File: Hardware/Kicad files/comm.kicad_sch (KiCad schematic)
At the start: 5 parts, among them J301 M80-5402642, J302 Conn_02x25_Top_Bottom, U301 MAX485_MODULE_5V_LOGIC_TLL_TO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

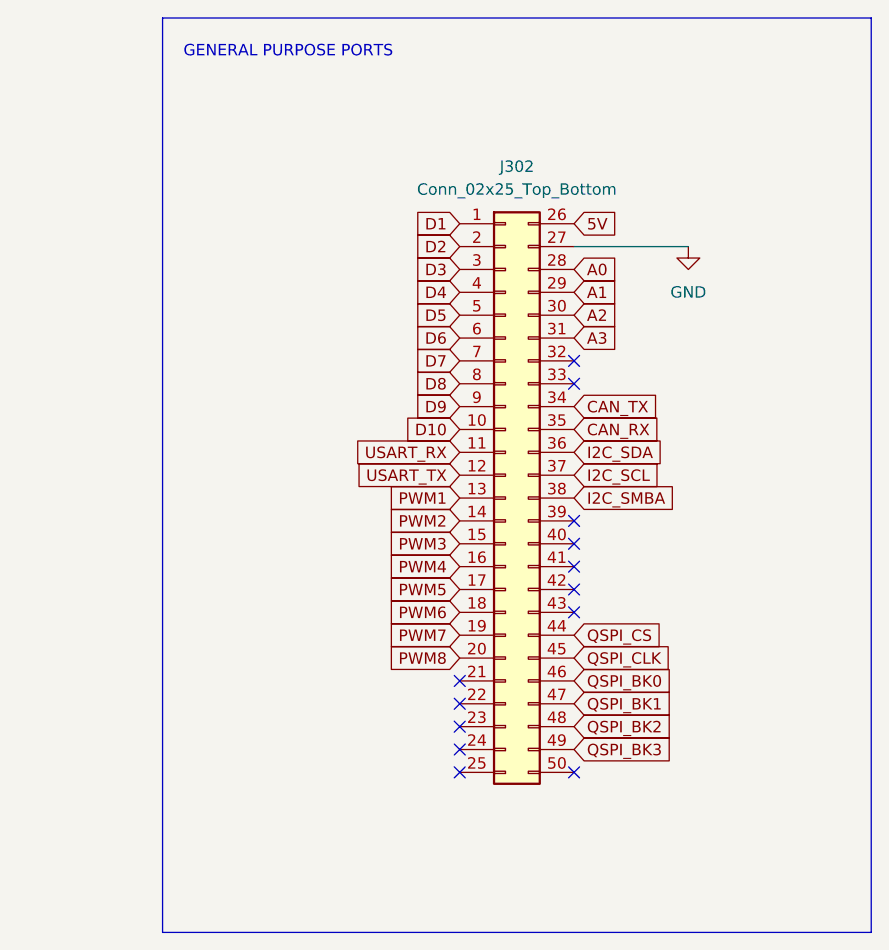
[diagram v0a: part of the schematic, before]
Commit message: Add files via upload
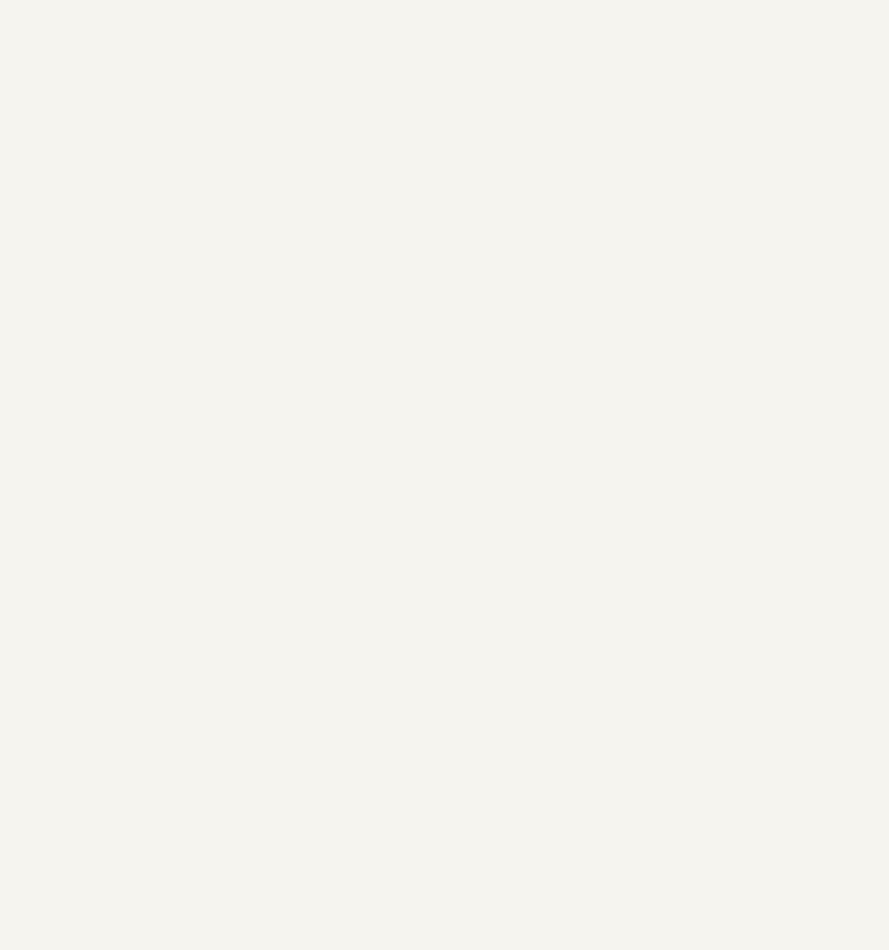
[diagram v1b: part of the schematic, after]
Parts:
- removed J302: Conn_02x25_Top_Bottom, Connector_PinSocket_2.54mm:PinSocket_2x25_P2.54mm_Vertical, symbol Connector_Generic:Conn_02x25_Top_Bottom
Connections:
- no-connect marks 29 -> 16
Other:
- note removed: "GENERAL PURPOSE PORTS"
